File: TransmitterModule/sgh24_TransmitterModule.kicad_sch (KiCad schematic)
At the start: 18 parts, among them J3 Battery, U1 NRF24L01_, U3 102010388

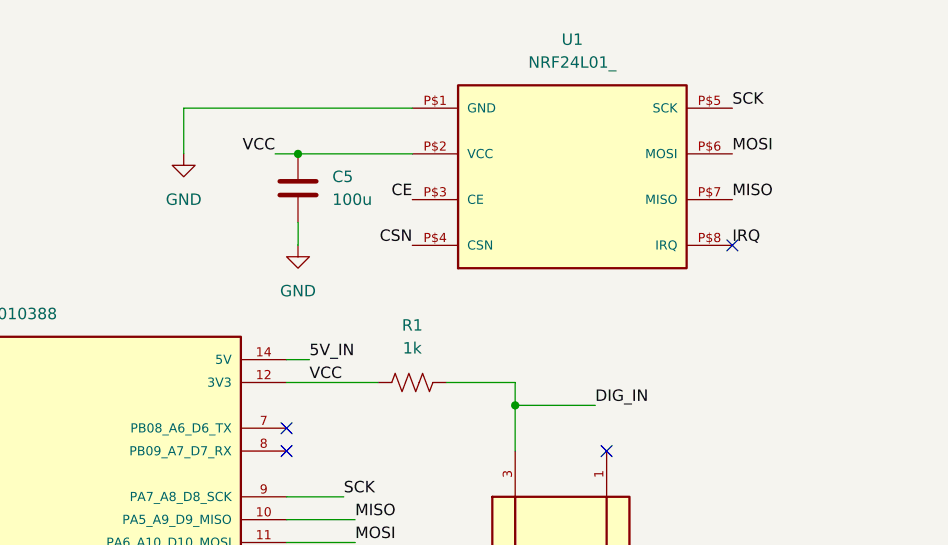
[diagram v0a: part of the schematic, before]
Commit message: added new firmware and pcb files
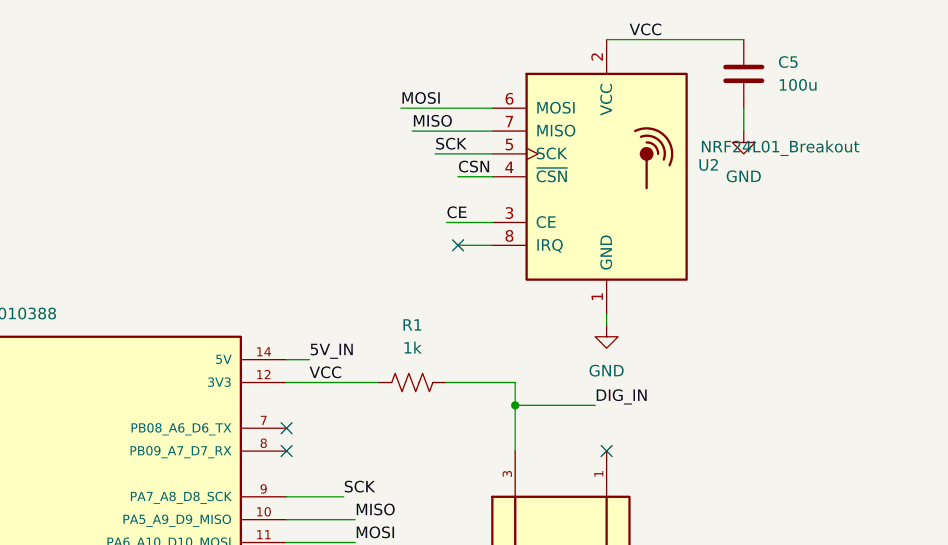
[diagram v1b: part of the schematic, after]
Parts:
- removed U1: NRF24L01_, RF_Module:nRF24L01_Breakout, symbol NRF24L01_:NRF24L01_
- added U2: NRF24L01_Breakout, RF_Module:nRF24L01_Breakout, symbol RF:NRF24L01_Breakout
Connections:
- net CE: now also U2.3 (CE)
- net CSN: now also U2.4 (~{CSN})
- net GND: now also U2.1 (GND)
- net MISO: now also U2.7 (MISO)
- net MOSI: now also U2.6 (MOSI)
- net SCK: now also U2.5 (SCK)
- net VCC: now also U2.2 (VCC)
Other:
- moved on the sheet: C5
